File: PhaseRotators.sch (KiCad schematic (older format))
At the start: 10 parts, among them U1 74LVC1G74, U2 74LVC74APW, U3 74LVC74APW, U4 74LVC1G74

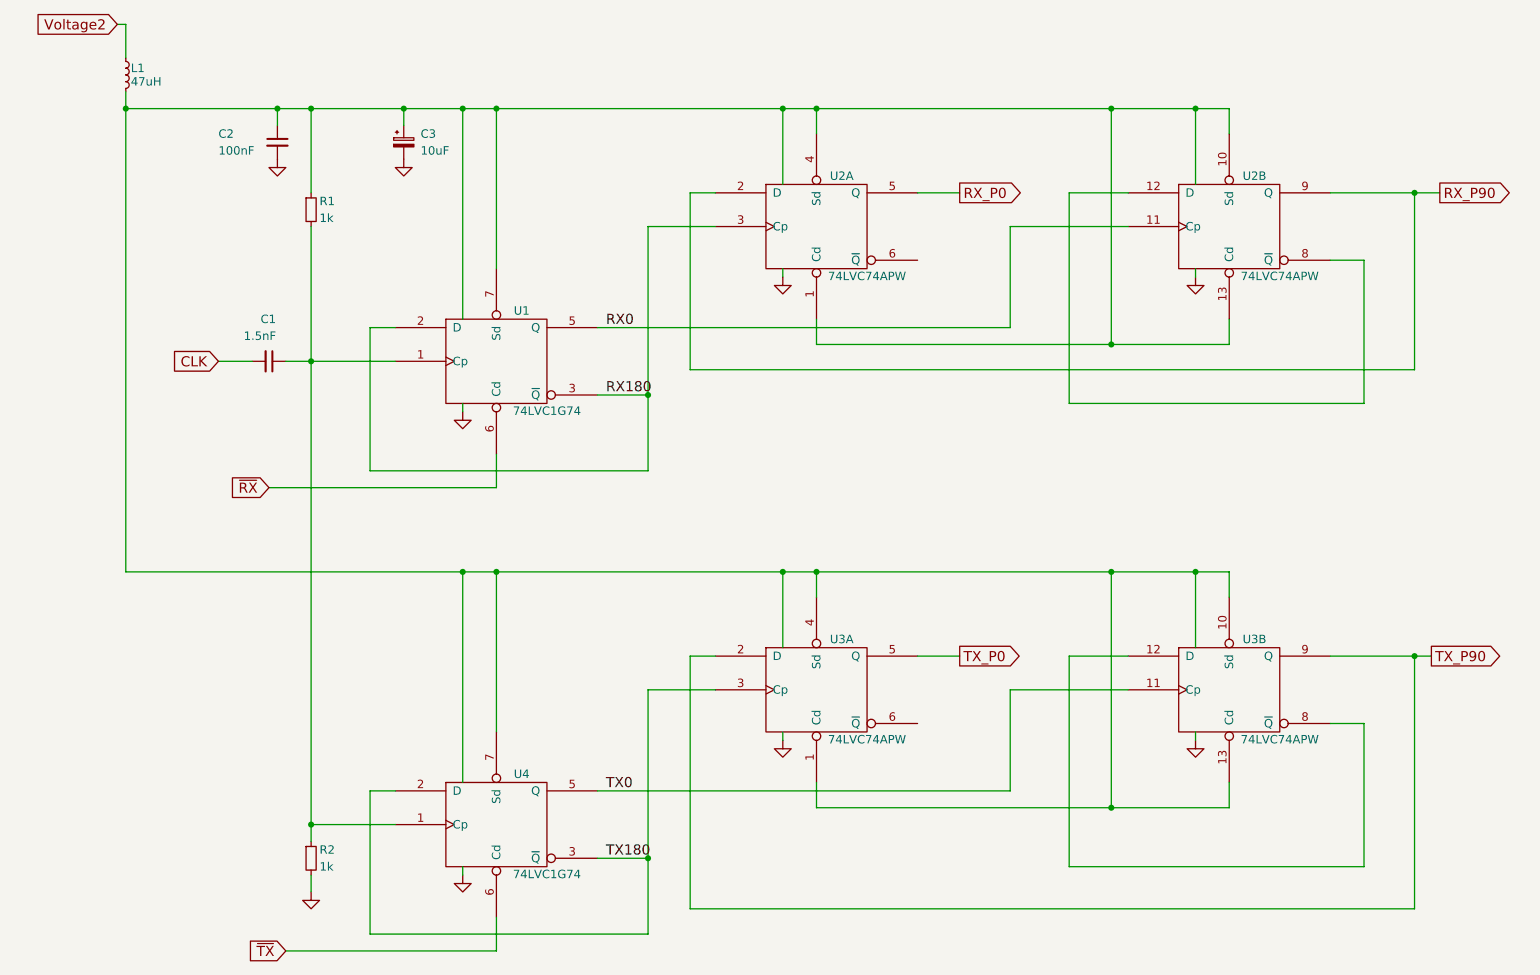
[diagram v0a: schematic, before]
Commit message: first edit
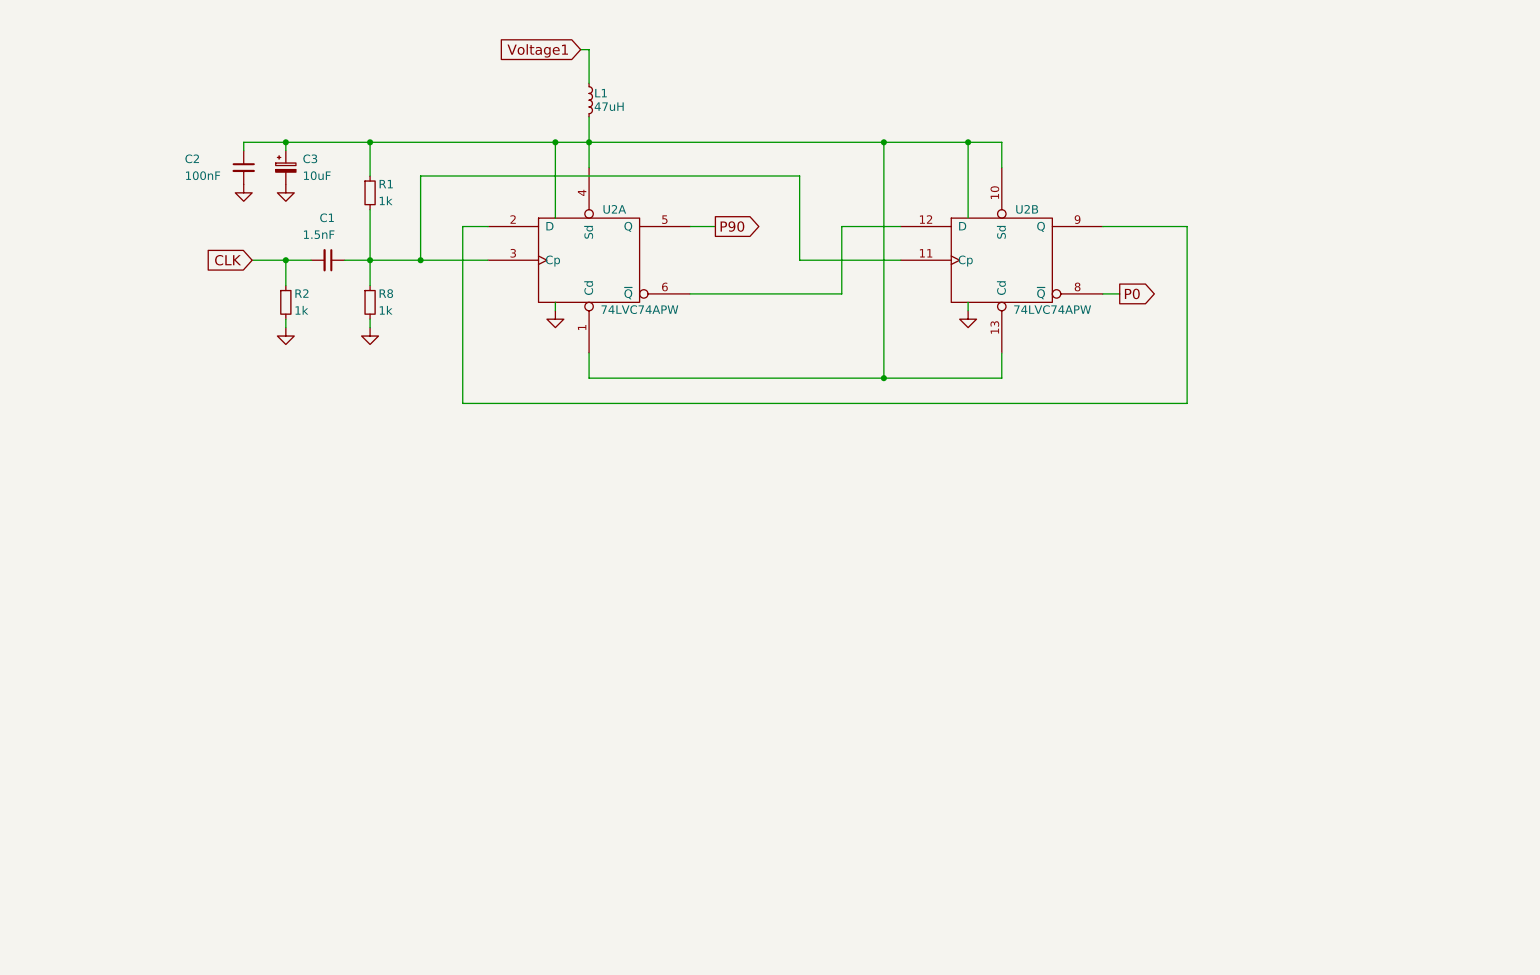
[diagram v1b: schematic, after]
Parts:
- removed U1, U4: 74LVC1G74, Housings_SSOP:TSSOP-8_3x3mm_Pitch0.65mm, symbol 74LVC1G74
- removed U3: 74LVC74APW, Housings_SSOP:TSSOP-14_4.4x5mm_Pitch0.65mm, symbol 74LS74
- added R8: 1k, Resistors_SMD:R_0603_HandSoldering, symbol R_Small
- C1, C2: footprint UI:C_1206_0603 -> Capacitors_SMD:C_0603_HandSoldering
- C3: footprint Capacitors_THT:CP_Radial_D5.0mm_P2.00mm -> Capacitors_Tantalum_SMD:CP_Tantalum_Case-A_EIA-3216-18_Wave
- L1: footprint Resistors_THT:R_Axial_DIN0207_L6.3mm_D2.5mm_P10.16mm_Horizontal -> Choke_Axial_ThroughHole:Choke_Horizontal_RM10mm
- R1, R2: footprint UI:R_1206_0603 -> Resistors_SMD:R_0603_HandSoldering
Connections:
- net RX0 is gone; now on an unnamed net: U2.11 (Cp)
- net RX180 is gone; now on an unnamed net: U2.3 (Cp)
- net CLK: now also R2.1
- net GND: now also R8.2
- net at U2.6 (~Q): now also U2.12 (D)
- net P0: now reaches U2.8 (~Q)
- net P0: no longer U2.12 (D)
- net at C1.1, R1.2: now also R8.1; no longer R2.1
- net RX_P0 renamed P90
- net RX_P90: no longer names the net of U2.2 (D), U2.9 (Q)
- net Voltage2 renamed Voltage1
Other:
- moved on the sheet: C1, C2, C3, L1, R1, U2A, U2B
